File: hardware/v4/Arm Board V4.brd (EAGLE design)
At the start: 108 x 50.8 mm, 38 parts, among them IC3 L6206D, P1 STELLARIS-LAUNCHPADSTELLARIS-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, U1 SN74LS241DW, U2 XBEE-1B3

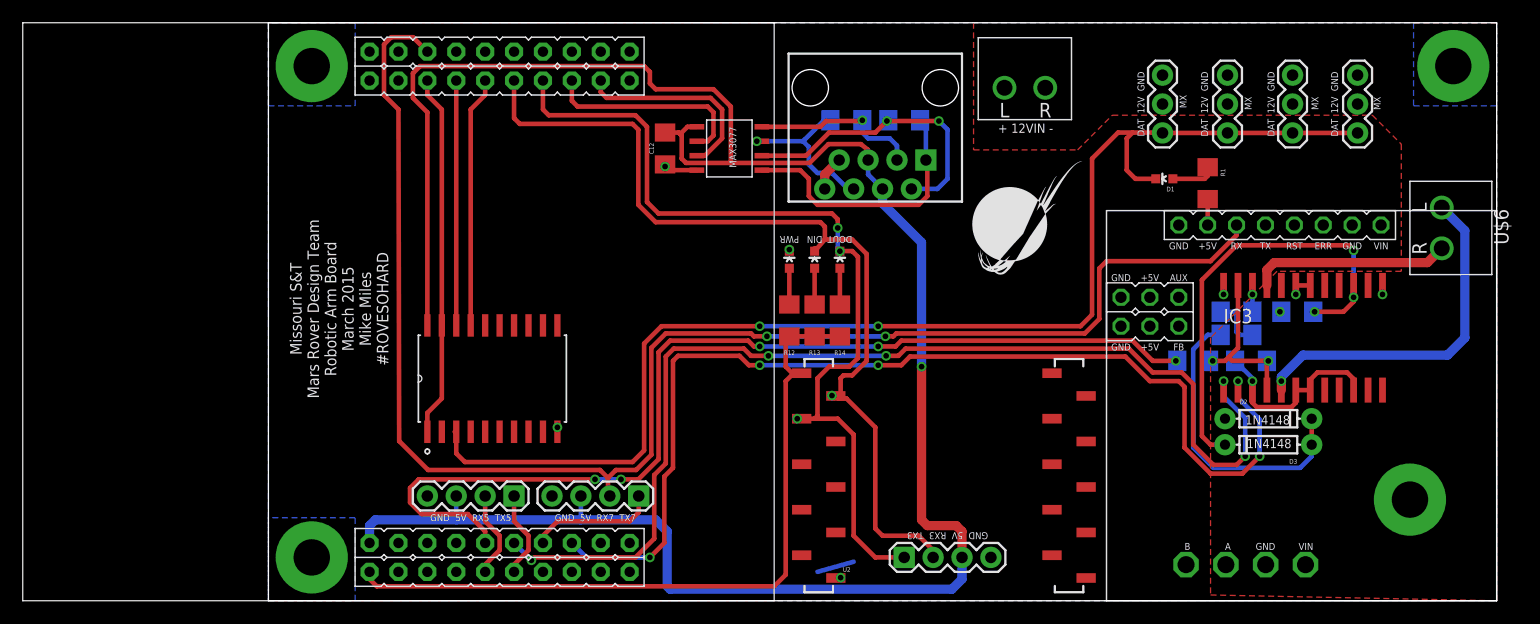
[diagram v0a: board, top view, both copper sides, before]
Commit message: about to reroute brd
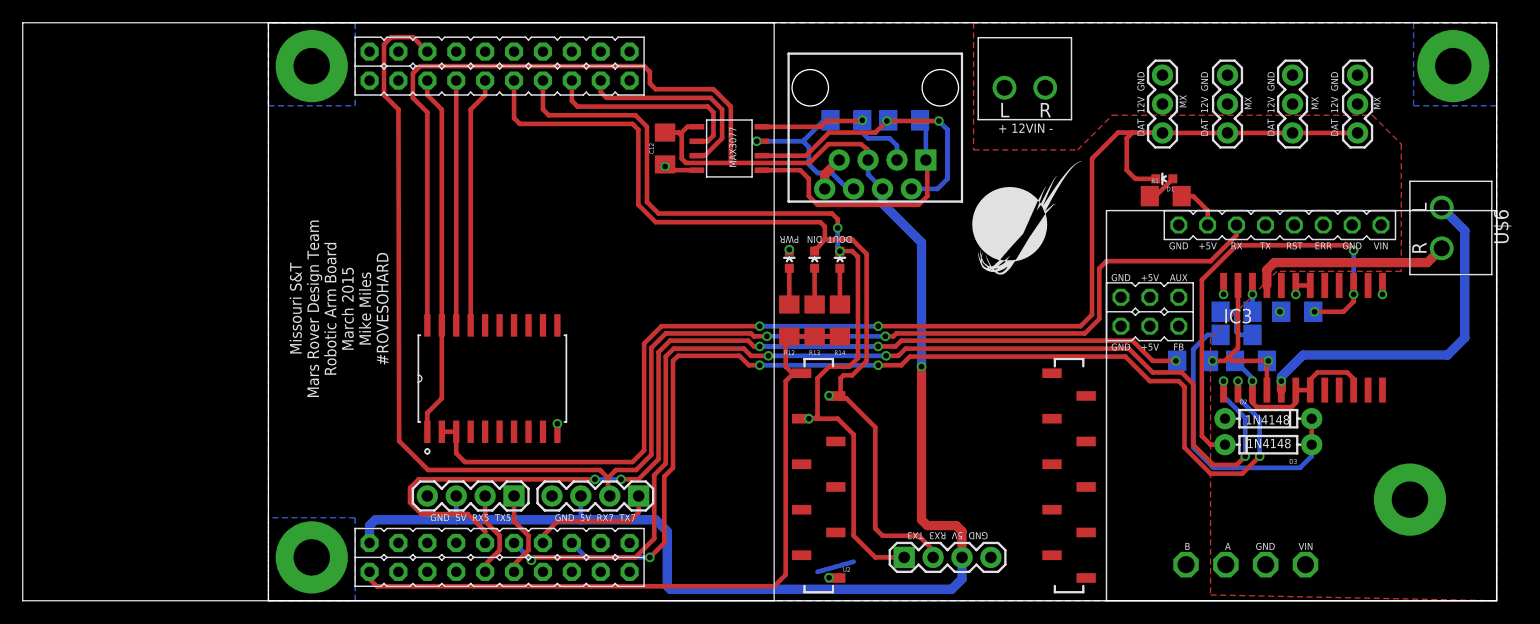
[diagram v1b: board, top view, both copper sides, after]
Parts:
- moved R1 3.86 mm to (78.9, 35.6), turned to 0 degrees
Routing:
- net +5V: track 189.4 -> 191.2 mm
- net N$13: track 3.93 -> 2.65 mm
- net DDATA_1: track 113.5 -> 114.7 mm
- net TX_3: track 77.5 -> 78.5 mm
- net RX_3: track 80.9 -> 81.6 mm
- net GND: track 31.2 -> 31.7 mm
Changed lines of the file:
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@@
 <layer number="21" name="tPlace" color="7" fill="1" visible="yes" active="yes"/>
 <layer number="22" name="bPlace" color="7" fill="1" visible="yes" active="yes"/>
-<layer number="23" name="tOrigins" color="15" fill="1" visible="no" active="yes"/>
-<layer number="24" name="bOrigins" color="15" fill="1" visible="no" active="yes"/>
+<layer number="23" name="tOrigins" color="15" fill="1" visible="yes" active="yes"/>
+<layer number="24" name="bOrigins" color="15" fill="1" visible="yes" active="yes"/>
 <layer number="25" name="tNames" color="7" fill="1" visible="no" active="yes"/>
 <layer number="26" name="bNames" color="7" fill="1" visible="no" active="yes"/>
@@
 </element>
 <element name="U$1" library="MRDT-RoboticArm" package="TORXIS_BREAKOUT" value="TORXIS_BREAKOUT" x="107.95" y="0" rot="R90"/>
-<element name="R1" library="SparkFun-Resistors" package="1206" value="1k" x="82.55" y="36.703" rot="R270"/>
+<element name="R1" library="SparkFun-Resistors" package="1206" value="1k" x="78.867" y="35.56"/>
 <element name="D1" library="SparkFun-LED" package="LED-0603" value="RED" x="78.74" y="37.084" rot="R90">
 <attribute name="PROD_ID" value="DIO-00819" x="78.74" y="37.084" size="1.778" layer="27" rot="R90" display="off"/>
@@
 <via x="34.8615" y="38.1635" extent="1-16" drill="0.5"/>
 <wire x1="34.8615" y1="38.351" x2="34.8615" y2="38.1635" width="0.4064" layer="1"/>
-<via x="25.4" y="15.24" extent="1-16" drill="0.5"/>
-<wire x1="25.4" y1="15.24" x2="25.4" y2="14.85265" width="0.4064" layer="1"/>
-<via x="50.292" y="2.032" extent="1-16" drill="0.5"/>
-<wire x1="50.292" y1="2.032" x2="49.902" y2="2.032" width="0.4064" layer="1"/>
+<via x="25.4" y="15.5575" extent="1-16" drill="0.5"/>
+<wire x1="25.4" y1="15.5575" x2="25.4" y2="14.85265" width="0.4064" layer="1"/>
+<via x="49.276" y="2.032" extent="1-16" drill="0.5"/>
+<wire x1="49.276" y1="2.032" x2="49.902" y2="2.032" width="0.4064" layer="1"/>
 <wire x1="49.902" y1="2.032" x2="49.87" y2="2" width="0.4064" layer="1"/>
 <wire x1="48.895" y1="36.195" x2="48.895" y2="37.465" width="0.8128" layer="1"/>
@@
 <contactref element="R1" pad="2"/>
 <contactref element="U$1" pad="+5V_OUT"/>
-<wire x1="82.55" y1="33.02" x2="82.55" y2="35.303" width="0.4064" layer="1"/>
 <wire x1="37.6555" y1="41.656" x2="36.83" y2="41.656" width="0.4064" layer="1"/>
 <wire x1="27.432" y1="9.23925" x2="27.432" y2="9.17575" width="0.4064" layer="16"/>
@@
 <wire x1="34.8645" y1="41.148" x2="34.8615" y2="41.151" width="0.4064" layer="1"/>
 <wire x1="36.83" y1="41.656" x2="36.195" y2="41.021" width="0.4064" layer="1"/>
-<wire x1="57.404" y1="31.496" x2="82.55" y2="33.02" width="0" layer="19" extent="16-16"/>
+<wire x1="82.55" y1="33.02" x2="82.55" y2="34.29" width="0.4064" layer="1"/>
+<wire x1="82.55" y1="34.29" x2="81.28" y2="35.56" width="0.4064" layer="1"/>
+<wire x1="81.28" y1="35.56" x2="80.267" y2="35.56" width="0.4064" layer="1"/>
+<wire x1="57.404" y1="31.496" x2="80.267" y2="35.56" width="0" layer="19" extent="1-16"/>
 </signal>
 <signal name="+12V">
@@
 <wire x1="49.65" y1="17.78" x2="49.87" y2="18" width="0.4064" layer="1"/>
 <wire x1="21.59" y1="45.72" x2="21.59" y2="42.418" width="0.4064" layer="1"/>
-<wire x1="49.53" y1="17.78" x2="49.53" y2="18.034" width="0.4064" layer="1"/>
-<via x="49.53" y="18.034" extent="1-16" drill="0.5"/>
+<wire x1="49.53" y1="17.78" x2="49.276" y2="18.034" width="0.4064" layer="1"/>
+<via x="49.276" y="18.034" extent="1-16" drill="0.5"/>
 <wire x1="22.098" y1="41.91" x2="21.59" y2="42.418" width="0.4064" layer="1"/>
 <wire x1="32.004" y1="41.91" x2="22.098" y2="41.91" width="0.4064" layer="1"/>
-<wire x1="49.784" y1="18.034" x2="49.53" y2="18.034" width="0.4064" layer="1"/>
-<wire x1="49.53" y1="18.034" x2="50.292" y2="18.034" width="0.4064" layer="1"/>
+<wire x1="49.784" y1="18.034" x2="49.276" y2="18.034" width="0.4064" layer="1"/>
+<wire x1="49.276" y1="18.034" x2="50.292" y2="18.034" width="0.4064" layer="1"/>
 <wire x1="50.292" y1="18.034" x2="50.292" y2="19.558" width="0.4064" layer="1"/>
 <wire x1="50.292" y1="19.558" x2="50.546" y2="19.812" width="0.4064" layer="1"/>
@@
 <wire x1="46.87" y1="16" x2="47.5" y2="16" width="0.4064" layer="1"/>
 <wire x1="46.87" y1="16" x2="46.484" y2="16" width="0.4064" layer="1"/>
-<wire x1="46.484" y1="16" x2="46.482" y2="16.002" width="0.4064" layer="1"/>
-<via x="46.482" y="16.002" extent="1-16" drill="0.5"/>
+<wire x1="46.484" y1="16" x2="47.498" y2="16.002" width="0.4064" layer="1"/>
+<via x="47.498" y="16.002" extent="1-16" drill="0.5"/>
 <wire x1="50.04" y1="16" x2="48.006" y2="16" width="0.4064" layer="1"/>
 <wire x1="48.006" y1="16" x2="47.5" y2="16" width="0.4064" layer="1"/>
@@
 <wire x1="75.438" y1="37.846" x2="75.438" y2="40.64" width="0.4064" layer="1"/>
 <wire x1="75.438" y1="40.64" x2="75.946" y2="41.148" width="0.4064" layer="1"/>
-<wire x1="16.38935" y1="14.85265" x2="15.24" y2="14.85265" width="0" layer="19" extent="1-1"/>
+<wire x1="16.38935" y1="14.85265" x2="15.24" y2="14.85265" width="0.4064" layer="1"/>
 </signal>
 <signal name="N$7">
@@
 <contactref element="R1" pad="1"/>
 <contactref element="D1" pad="A"/>
-<wire x1="82.55" y1="38.103" x2="82.55" y2="37.338" width="0.4064" layer="1"/>
-<wire x1="82.55" y1="37.338" x2="82.296" y2="37.084" width="0.4064" layer="1"/>
-<wire x1="82.296" y1="37.084" x2="79.49" y2="37.084" width="0.4064" layer="1"/>
+<wire x1="77.467" y1="35.56" x2="77.966" y2="35.56" width="0.4064" layer="1"/>
+<wire x1="77.966" y1="35.56" x2="79.49" y2="37.084" width="0.4064" layer="1"/>
 </signal>
 <signal name="A1">
@@
 <contactref element="IC3" pad="15"/>
 <via x="91.948" y="25.4" extent="1-16" drill="0.5"/>
-<wire x1="95.377" y1="27.714" x2="95.377" y2="26.67" width="0.4064" layer="1"/>
-<wire x1="95.377" y1="26.67" x2="95.377" y2="26.289" width="0.4064" layer="1"/>
+<wire x1="95.377" y1="27.714" x2="95.377" y2="26.924" width="0.4064" layer="1"/>
+<wire x1="95.377" y1="26.924" x2="95.377" y2="26.289" width="0.4064" layer="1"/>
 <wire x1="95.377" y1="26.289" x2="94.488" y2="25.4" width="0.4064" layer="1"/>
 <wire x1="94.488" y1="25.4" x2="91.948" y2="25.4" width="0.4064" layer="1"/>
@@
 <wire x1="94.9325" y1="31.242" x2="95.377" y2="30.7975" width="0.4064" layer="1"/>
 <via x="95.377" y="30.7975" extent="1-16" drill="0.5"/>
-<wire x1="95.377" y1="30.7975" x2="95.377" y2="26.67" width="0.4064" layer="16"/>
-<via x="95.377" y="26.67" extent="1-16" drill="0.5"/>
+<wire x1="95.377" y1="30.7975" x2="95.377" y2="26.924" width="0.4064" layer="16"/>
+<via x="95.377" y="26.924" extent="1-16" drill="0.5"/>
 </signal>
 </signals>

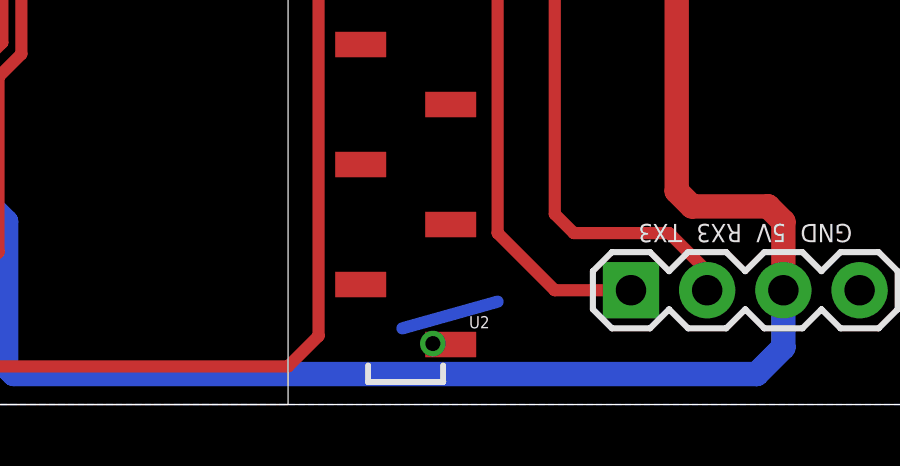
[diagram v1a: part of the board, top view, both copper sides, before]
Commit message: didnt do much
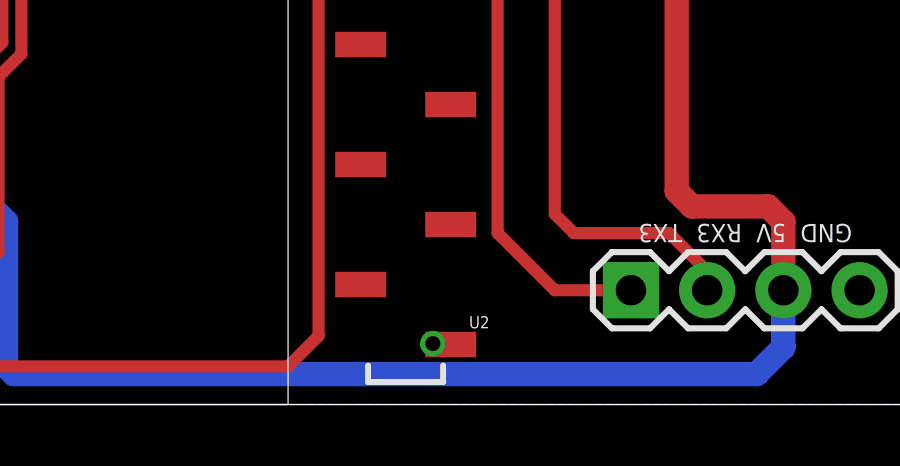
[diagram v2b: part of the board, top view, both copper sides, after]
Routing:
- net GND: track 31.7 -> 28.4 mm
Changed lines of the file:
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@@
 </polygon>
 <wire x1="49.87" y1="2" x2="50.006" y2="2" width="0.4064" layer="1"/>
-<wire x1="51.435" y1="3.429" x2="48.26" y2="2.54" width="0.4064" layer="16"/>
 <via x="45.7835" y="30.861" extent="1-16" drill="0.5"/>
 <wire x1="37.6555" y1="37.846" x2="35.3665" y2="37.846" width="0.4064" layer="1"/>
